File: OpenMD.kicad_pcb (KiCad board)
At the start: 4 copper layers, 80 x 50 mm, 167 parts, among them IC2 RAA2118054GP3#JA0, J1 GND, J2 Digital, J3 Analog, J4 Sensors, J5 A, J6 B, J7 C, J8 V_{BATT}, Q1 EPC2065, Q2 EPC2065, Q3 EPC2065, Q7 EPC2065, Q8 EPC2065, Q9 EPC2065, U1 UP1966E, U10 INA240A2, U2 UP1966E, U3 UP1966E, U8 INA240A2, U9 INA240A2

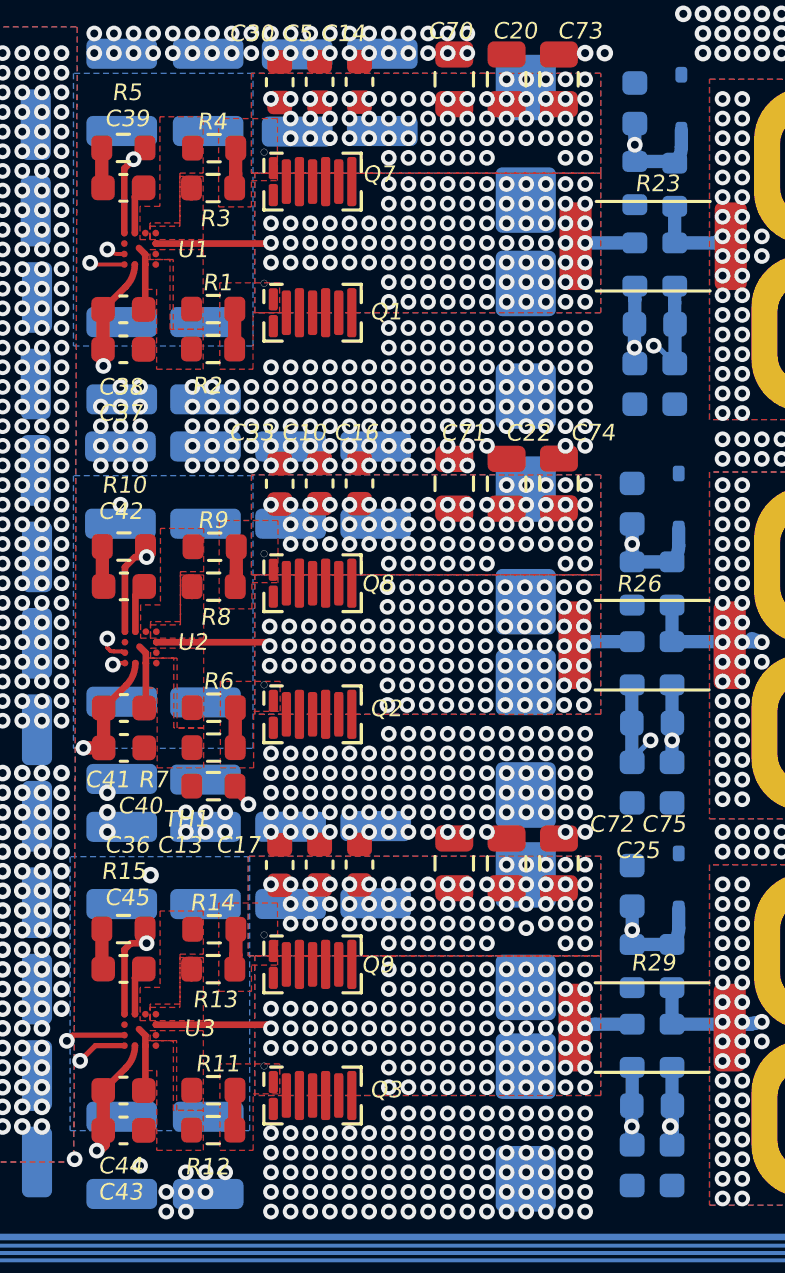
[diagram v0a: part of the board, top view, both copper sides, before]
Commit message: added docs
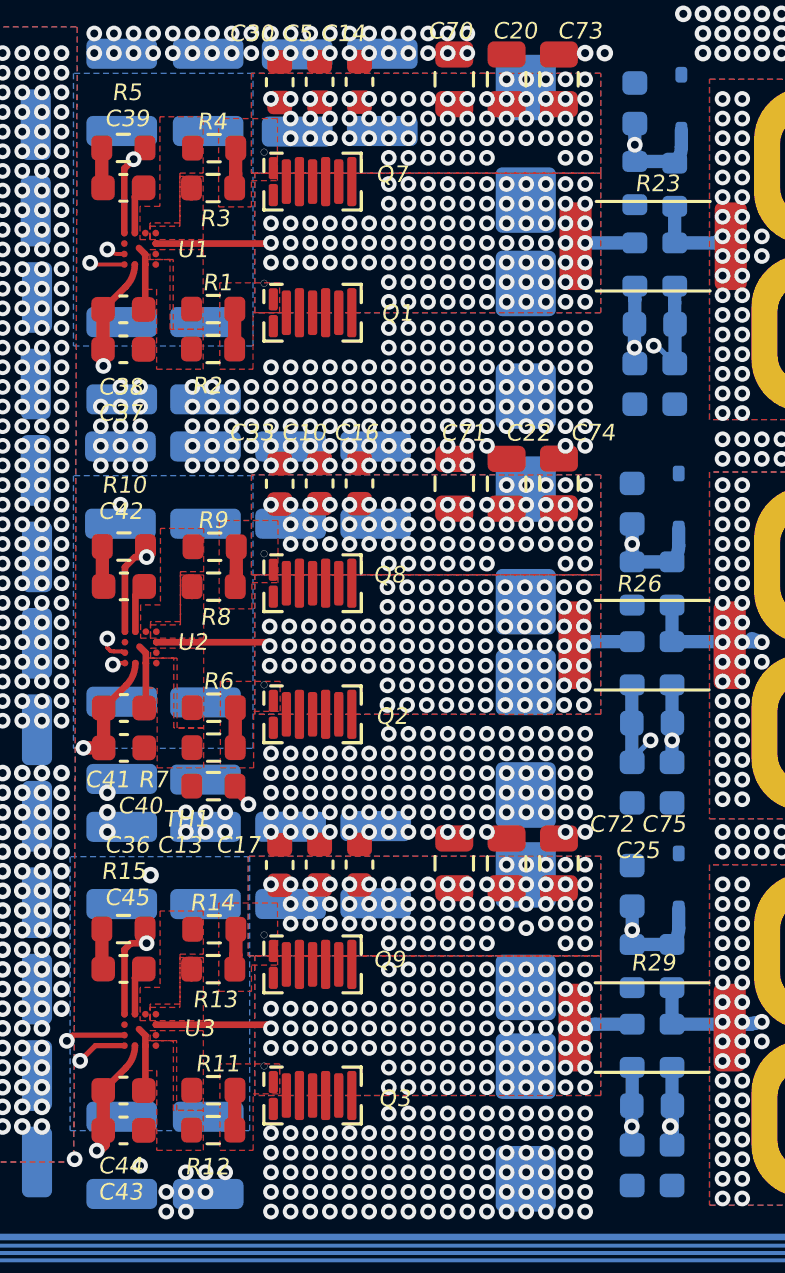
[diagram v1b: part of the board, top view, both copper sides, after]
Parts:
- IC2: value RAA2118054GP3#JA0 -> RAA211
